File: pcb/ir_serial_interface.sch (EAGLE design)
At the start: 24 parts, among them IC1 PIC18F2550_28W, Q1 BSS123, T1 SFH303

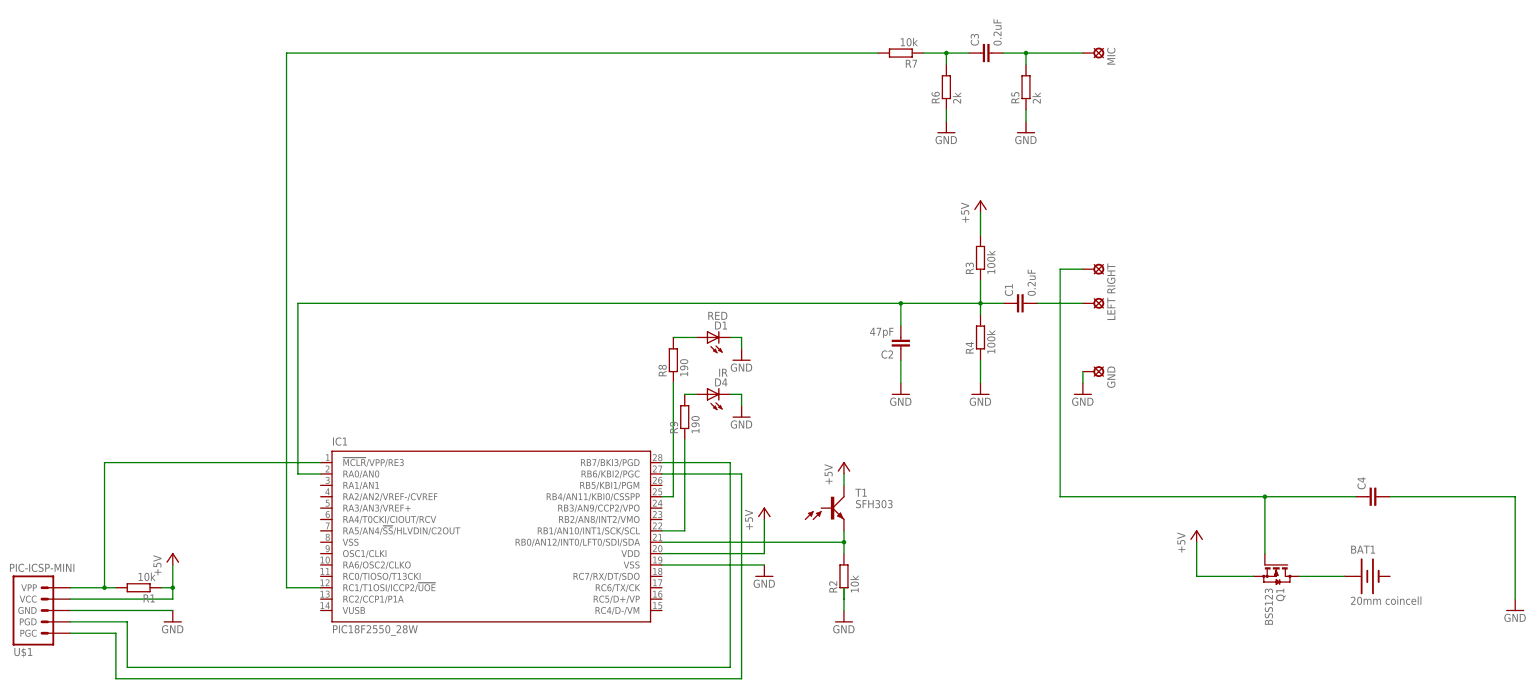
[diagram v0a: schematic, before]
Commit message: PCB: board layout done
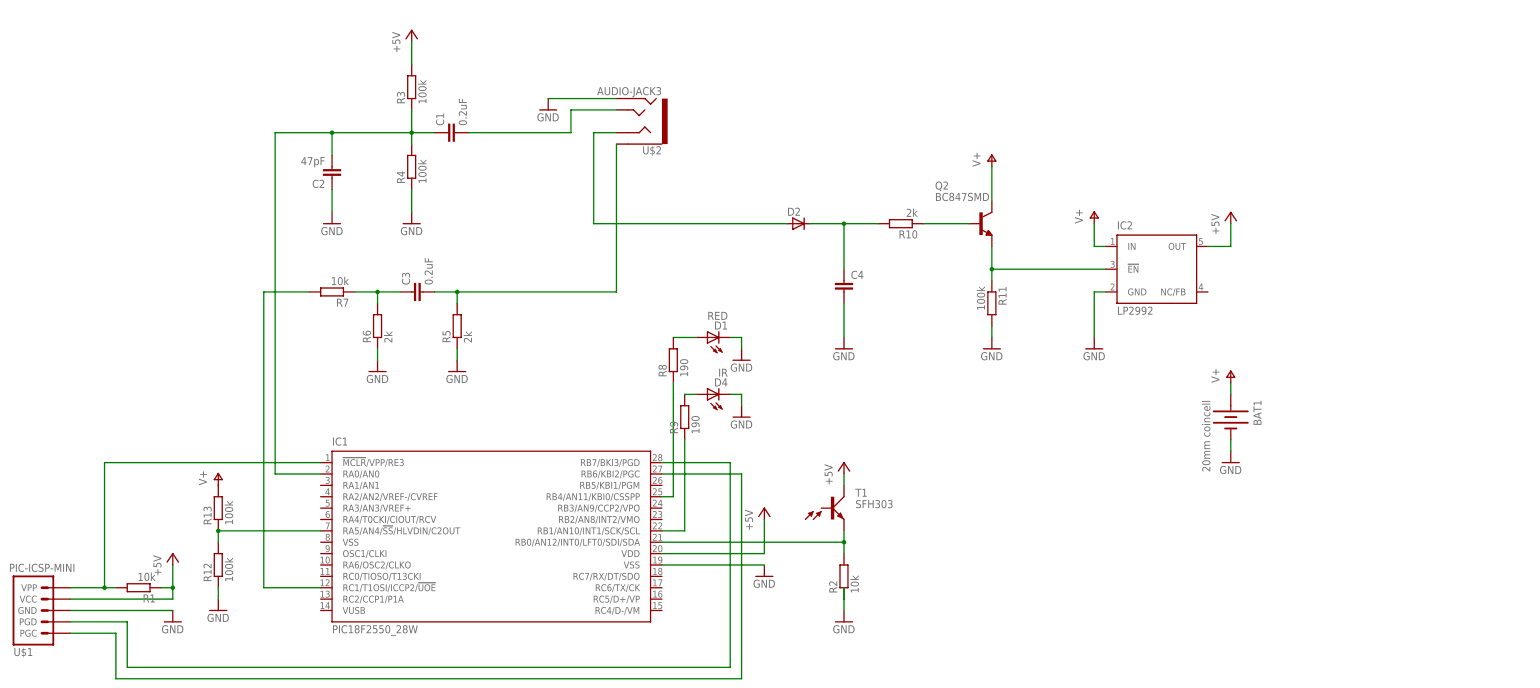
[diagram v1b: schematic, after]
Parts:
- removed GND, LEFT, MIC, RIGHT: LSP10, solpad:LSP10
- removed Q1: BSS123, transistor-small-signal:BSS123
- added D2: (no value), semicon-smd-ipc:D-A1-C3
- added IC2: LP2992, texas:TPS77001
- added Q2: BC847SMD, transistor-npn:BC847SMD
- added R10: 2k, resistor:R-EU_M0805
- added R11, R12, R13: 100k, resistor:R-EU_M0805
- added U$2: AUDIO-JACK3, SparkFun-Connectors:AUDIO-JACK3
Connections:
- new net N$12: D2.A, U$2.RING1
- new net N$13: IC2.!EN, Q2.E, R11.1
- new net N$18: C4.1, D2.C, R10.2
- new net V+: BAT1.+, IC2.IN, Q2.C, R13.2
- net +5V: now also IC2.OUT; no longer Q1.S
- net GND: now also BAT1.-, IC2.GND, R11.2, R12.1, U$2.RING2; no longer GND.MP
- net N$16: now also IC1.RA5/AN4/!SS!/HLVDIN/C2OUT, R12.2, R13.1; no longer BAT1.+, Q1.D
- net N$17: now also Q2.B, R10.1; no longer C4.1, Q1.G, RIGHT.MP
- net N$5: now also U$2.TIP; no longer LEFT.MP
- net N$7: now also U$2.EARTH; no longer MIC.MP
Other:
- moved on the sheet: BAT1, C1, C2, C3, C4, R3, R4, R5, R6, R7
